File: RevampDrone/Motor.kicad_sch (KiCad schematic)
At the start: 5 parts, among them J3 Conn_02x03_Counter_Clockwise, J4 Conn_02x03_Counter_Clockwise, J5 Conn_02x03_Counter_Clockwise, J6 Conn_02x03_Counter_Clockwise, U10 PCA9531PW

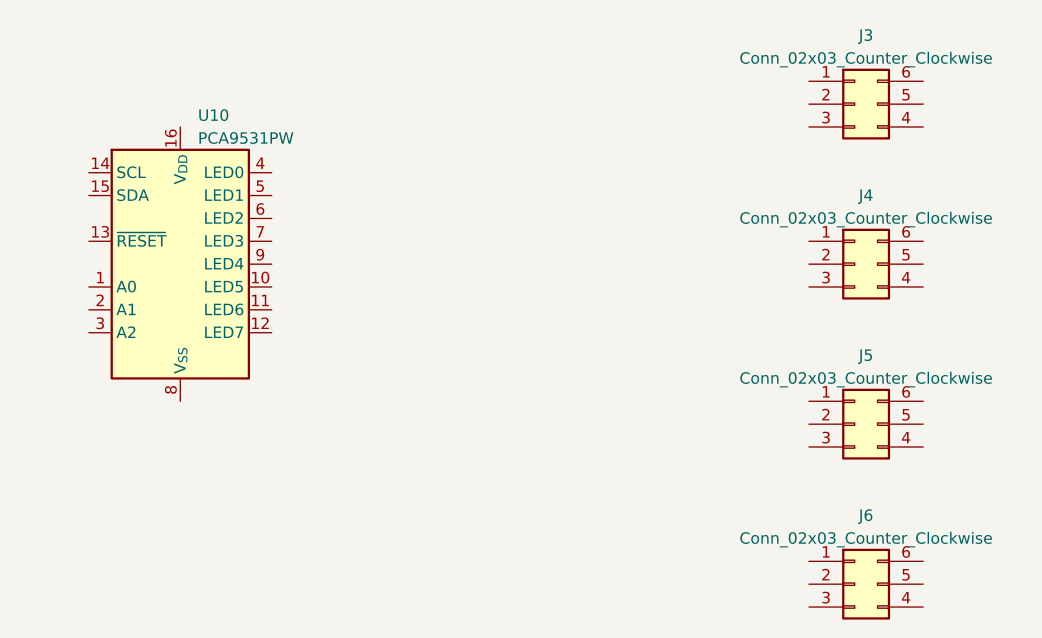
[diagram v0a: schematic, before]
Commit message: Get it on V7
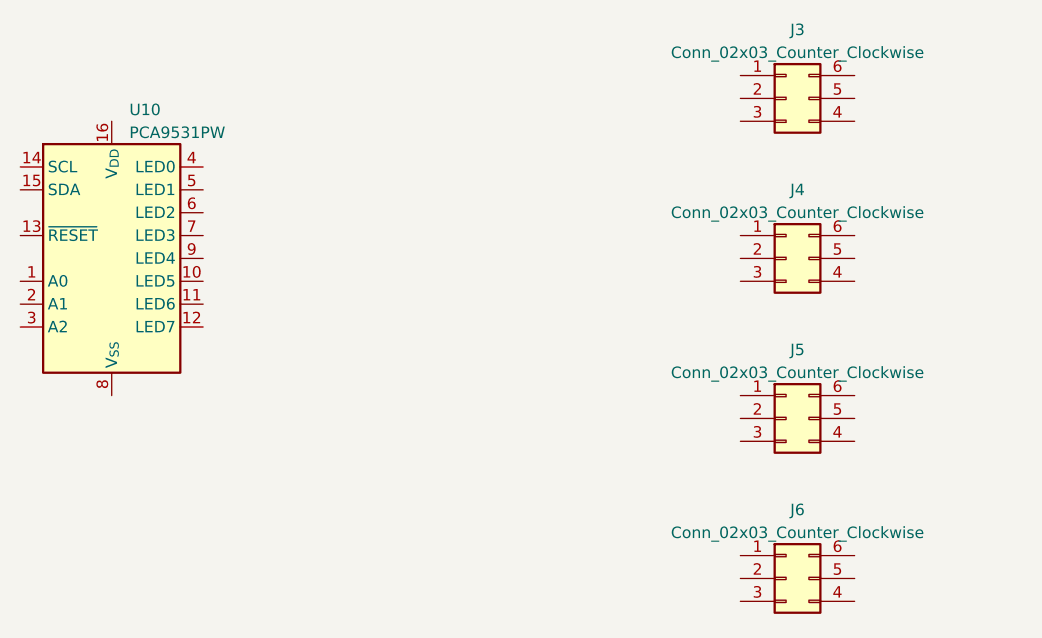
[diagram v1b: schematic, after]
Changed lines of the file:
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@@
 (kicad_sch (version 20230121) (generator eeschema)
   (paper "A4")
-  (symbol (lib_id "Connector_Generic:Conn_02x03_Counter_Clockwise") (at 168.275 99.06 0) (unit 1)
-    (in_bom yes) (on_board yes) (dnp no) (fields_autoplaced)
-    (property "Reference" "J5" (at 169.545 91.44 0)
-      (effects (font (size 1.27 1.27)))
-    )
-    (property "Value" "Conn_02x03_Counter_Clockwise" (at 169.545 93.98 0)
-      (effects (font (size 1.27 1.27)))
-    )
-    (property "Footprint" "" (at 168.275 99.06 0)
-      (effects (font (size 1.27 1.27)) hide)
-    )
-    (property "Datasheet" "~" (at 168.275 99.06 0)
-      (effects (font (size 1.27 1.27)) hide)
-    )
-    (pin "1")
-    (pin "2")
-    (pin "3")
-    (pin "4")
-    (pin "5")
-    (pin "6")
-    (instances
-      (project "DroneRevamp"
-        (path "/b197cc17-7ac5-409f-9705-26347f5a482b/37bf618c-4148-4ee8-8976-266644a9d57f"
-          (reference "J5") (unit 1)
-        )
-      )
-    )
-  )
-  (symbol (lib_id "Driver_LED:PCA9531PW") (at 93.345 81.28 0) (unit 1)
-    (in_bom yes) (on_board yes) (dnp no) (fields_autoplaced)
-    (property "Reference" "U10" (at 95.3009 64.77 0)
+  (symbol (lib_id "Driver_LED:PCA9531PW") (at 85.725 80.645 0) (unit 1)
+    (in_bom yes) (on_board yes) (dnp no) (fields_autoplaced)
+    (property "Reference" "U10" (at 87.6809 64.135 0)
       (effects (font (size 1.27 1.27)) (justify left))
     )
-    (property "Value" "PCA9531PW" (at 95.3009 67.31 0)
+    (property "Value" "PCA9531PW" (at 87.6809 66.675 0)
       (effects (font (size 1.27 1.27)) (justify left))
     )
-    (property "Footprint" "Package_SO:TSSOP-16_4.4x5mm_P0.65mm" (at 93.345 83.82 0)
-      (effects (font (size 1.27 1.27)) hide)
-    )
-    (property "Datasheet" "https://www.nxp.com/docs/en/data-sheet/PCA9531.pdf" (at 93.345 83.82 0)
+    (property "Footprint" "Package_SO:TSSOP-16_4.4x5mm_P0.65mm" (at 85.725 83.185 0)
+      (effects (font (size 1.27 1.27)) hide)
+    )
+    (property "Datasheet" "https://www.nxp.com/docs/en/data-sheet/PCA9531.pdf" (at 85.725 83.185 0)
       (effects (font (size 1.27 1.27)) hide)
     )
@@
     (pin "9")
     (instances
+      (project "Motors"
+        (path "/1535f15a-de4f-4945-863b-f274f44bb24c"
+          (reference "U10") (unit 1)
+        )
+      )
+      (project "RevampDrone"
+        (path "/a57dd8a7-b3ae-4be1-9fc6-9c9c7e0e2ba9/5515ab7f-03a0-465d-b71f-0a18b532a6c5"
+          (reference "U10") (unit 1)
+        )
+      )
       (project "DroneRevamp"
         (path "/b197cc17-7ac5-409f-9705-26347f5a482b/cd60092a-1d91-439d-a55b-26434dc4780f"
@@
     )
   )
-  (symbol (lib_id "Connector_Generic:Conn_02x03_Counter_Clockwise") (at 168.275 63.5 0) (unit 1)
-    (in_bom yes) (on_board yes) (dnp no) (fields_autoplaced)
-    (property "Reference" "J3" (at 169.545 55.88 0)
-      (effects (font (size 1.27 1.27)))
-    )
-    (property "Value" "Conn_02x03_Counter_Clockwise" (at 169.545 58.42 0)
-      (effects (font (size 1.27 1.27)))
-    )
-    (property "Footprint" "" (at 168.275 63.5 0)
-      (effects (font (size 1.27 1.27)) hide)
-    )
-    (property "Datasheet" "~" (at 168.275 63.5 0)
-      (effects (font (size 1.27 1.27)) hide)
-    )
-    (pin "1")
-    (pin "2")
-    (pin "3")
-    (pin "4")
-    (pin "5")
-    (pin "6")
-    (instances
-      (project "DroneRevamp"
-        (path "/b197cc17-7ac5-409f-9705-26347f5a482b/37bf618c-4148-4ee8-8976-266644a9d57f"
+  (symbol (lib_id "Connector_Generic:Conn_02x03_Counter_Clockwise") (at 160.655 98.425 0) (unit 1)
+    (in_bom yes) (on_board yes) (dnp no) (fields_autoplaced)
+    (property "Reference" "J5" (at 161.925 90.805 0)
+      (effects (font (size 1.27 1.27)))
+    )
+    (property "Value" "Conn_02x03_Counter_Clockwise" (at 161.925 93.345 0)
+      (effects (font (size 1.27 1.27)))
+    )
+    (property "Footprint" "" (at 160.655 98.425 0)
+      (effects (font (size 1.27 1.27)) hide)
+    )
+    (property "Datasheet" "~" (at 160.655 98.425 0)
+      (effects (font (size 1.27 1.27)) hide)
+    )
+    (pin "1")
+    (pin "2")
+    (pin "3")
+    (pin "4")
+    (pin "5")
+    (pin "6")
+    (instances
+      (project "Motors"
+        (path "/1535f15a-de4f-4945-863b-f274f44bb24c"
+          (reference "J5") (unit 1)
+        )
+      )
+      (project "RevampDrone"
+        (path "/a57dd8a7-b3ae-4be1-9fc6-9c9c7e0e2ba9/5515ab7f-03a0-465d-b71f-0a18b532a6c5"
+          (reference "J5") (unit 1)
+        )
+      )
+      (project "DroneRevamp"
+        (path "/b197cc17-7ac5-409f-9705-26347f5a482b/37bf618c-4148-4ee8-8976-266644a9d57f"
+          (reference "J5") (unit 1)
+        )
+      )
+    )
+  )
+  (symbol (lib_id "Connector_Generic:Conn_02x03_Counter_Clockwise") (at 160.655 62.865 0) (unit 1)
+    (in_bom yes) (on_board yes) (dnp no) (fields_autoplaced)
+    (property "Reference" "J3" (at 161.925 55.245 0)
+      (effects (font (size 1.27 1.27)))
+    )
+    (property "Value" "Conn_02x03_Counter_Clockwise" (at 161.925 57.785 0)
+      (effects (font (size 1.27 1.27)))
+    )
+    (property "Footprint" "" (at 160.655 62.865 0)
+      (effects (font (size 1.27 1.27)) hide)
+    )
+    (property "Datasheet" "~" (at 160.655 62.865 0)
+      (effects (font (size 1.27 1.27)) hide)
+    )
+    (pin "1")
+    (pin "2")
+    (pin "3")
+    (pin "4")
+    (pin "5")
+    (pin "6")
+    (instances
+      (project "Motors"
+        (path "/1535f15a-de4f-4945-863b-f274f44bb24c"
           (reference "J3") (unit 1)
         )
       )
-    )
-  )
-  (symbol (lib_id "Connector_Generic:Conn_02x03_Counter_Clockwise") (at 168.275 116.84 0) (unit 1)
-    (in_bom yes) (on_board yes) (dnp no) (fields_autoplaced)
-    (property "Reference" "J6" (at 169.545 109.22 0)
-      (effects (font (size 1.27 1.27)))
-    )
-    (property "Value" "Conn_02x03_Counter_Clockwise" (at 169.545 111.76 0)
-      (effects (font (size 1.27 1.27)))
-    )
-    (property "Footprint" "" (at 168.275 116.84 0)
-      (effects (font (size 1.27 1.27)) hide)
-    )
-    (property "Datasheet" "~" (at 168.275 116.84 0)
-      (effects (font (size 1.27 1.27)) hide)
-    )
-    (pin "1")
-    (pin "2")
-    (pin "3")
-    (pin "4")
-    (pin "5")
-    (pin "6")
-    (instances
-      (project "DroneRevamp"
-        (path "/b197cc17-7ac5-409f-9705-26347f5a482b/37bf618c-4148-4ee8-8976-266644a9d57f"
+      (project "RevampDrone"
+        (path "/a57dd8a7-b3ae-4be1-9fc6-9c9c7e0e2ba9/5515ab7f-03a0-465d-b71f-0a18b532a6c5"
+          (reference "J3") (unit 1)
+        )
+      )
+      (project "DroneRevamp"
+        (path "/b197cc17-7ac5-409f-9705-26347f5a482b/37bf618c-4148-4ee8-8976-266644a9d57f"
+          (reference "J3") (unit 1)
+        )
+      )
+    )
+  )
+  (symbol (lib_id "Connector_Generic:Conn_02x03_Counter_Clockwise") (at 160.655 116.205 0) (unit 1)
+    (in_bom yes) (on_board yes) (dnp no) (fields_autoplaced)
+    (property "Reference" "J6" (at 161.925 108.585 0)
+      (effects (font (size 1.27 1.27)))
+    )
+    (property "Value" "Conn_02x03_Counter_Clockwise" (at 161.925 111.125 0)
+      (effects (font (size 1.27 1.27)))
+    )
+    (property "Footprint" "" (at 160.655 116.205 0)
+      (effects (font (size 1.27 1.27)) hide)
+    )
+    (property "Datasheet" "~" (at 160.655 116.205 0)
+      (effects (font (size 1.27 1.27)) hide)
+    )
+    (pin "1")
+    (pin "2")
+    (pin "3")
+    (pin "4")
+    (pin "5")
+    (pin "6")
+    (instances
+      (project "Motors"
+        (path "/1535f15a-de4f-4945-863b-f274f44bb24c"
           (reference "J6") (unit 1)
         )
       )
-    )
-  )
-  (symbol (lib_id "Connector_Generic:Conn_02x03_Counter_Clockwise") (at 168.275 81.28 0) (unit 1)
-    (in_bom yes) (on_board yes) (dnp no) (fields_autoplaced)
-    (property "Reference" "J4" (at 169.545 73.66 0)
-      (effects (font (size 1.27 1.27)))
-    )
-    (property "Value" "Conn_02x03_Counter_Clockwise" (at 169.545 76.2 0)
-      (effects (font (size 1.27 1.27)))
-    )
-    (property "Footprint" "" (at 168.275 81.28 0)
-      (effects (font (size 1.27 1.27)) hide)
-    )
-    (property "Datasheet" "~" (at 168.275 81.28 0)
-      (effects (font (size 1.27 1.27)) hide)
-    )
-    (pin "1")
-    (pin "2")
-    (pin "3")
-    (pin "4")
-    (pin "5")
-    (pin "6")
-    (instances
-      (project "DroneRevamp"
-        (path "/b197cc17-7ac5-409f-9705-26347f5a482b/37bf618c-4148-4ee8-8976-266644a9d57f"
+      (project "RevampDrone"
+        (path "/a57dd8a7-b3ae-4be1-9fc6-9c9c7e0e2ba9/5515ab7f-03a0-465d-b71f-0a18b532a6c5"
+          (reference "J6") (unit 1)
+        )
+      )
+      (project "DroneRevamp"
+        (path "/b197cc17-7ac5-409f-9705-26347f5a482b/37bf618c-4148-4ee8-8976-266644a9d57f"
+          (reference "J6") (unit 1)
+        )
+      )
+    )
+  )
+  (symbol (lib_id "Connector_Generic:Conn_02x03_Counter_Clockwise") (at 160.655 80.645 0) (unit 1)
+    (in_bom yes) (on_board yes) (dnp no) (fields_autoplaced)
+    (property "Reference" "J4" (at 161.925 73.025 0)
+      (effects (font (size 1.27 1.27)))
+    )
+    (property "Value" "Conn_02x03_Counter_Clockwise" (at 161.925 75.565 0)
+      (effects (font (size 1.27 1.27)))
+    )
+    (property "Footprint" "" (at 160.655 80.645 0)
+      (effects (font (size 1.27 1.27)) hide)
+    )
+    (property "Datasheet" "~" (at 160.655 80.645 0)
+      (effects (font (size 1.27 1.27)) hide)
+    )
+    (pin "1")
+    (pin "2")
+    (pin "3")
+    (pin "4")
+    (pin "5")
+    (pin "6")
+    (instances
+      (project "Motors"
+        (path "/1535f15a-de4f-4945-863b-f274f44bb24c"
+          (reference "J4") (unit 1)
+        )
+      )
+      (project "RevampDrone"
+        (path "/a57dd8a7-b3ae-4be1-9fc6-9c9c7e0e2ba9/5515ab7f-03a0-465d-b71f-0a18b532a6c5"
+          (reference "J4") (unit 1)
+        )
+      )
+      (project "DroneRevamp"
+        (path "/b197cc17-7ac5-409f-9705-26347f5a482b/37bf618c-4148-4ee8-8976-266644a9d57f"
